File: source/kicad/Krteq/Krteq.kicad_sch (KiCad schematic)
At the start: 137 parts, among them J71 OLED 128x32, SW1 Switch, SW10 Switch, SW11 Switch, SW12 Switch, SW13 Switch, SW14 Switch, SW15 Switch, SW16 Switch, SW17 Switch, SW18 Switch, SW19 Switch, SW2 Switch, SW20 Switch, SW21 Switch, SW22 Switch, SW23 Switch, SW24 Switch, SW25 Switch, SW26 Switch, SW27 Switch, SW28 Switch, SW29 Switch, SW3 Switch, SW30 Switch, SW31 Switch, SW32 Switch, SW33 Switch, SW34 Switch, SW35 Switch, SW36 Switch, SW37 Switch, SW38 Switch, SW39 Switch, SW4 Switch, SW40 Switch, SW41 Switch, SW42 Switch, SW43 Switch, SW44 Switch, SW45 Switch, SW46 Switch, SW47 Switch, SW48 Switch, SW49 Switch, SW5 Switch, SW50 Switch, SW51 Switch, SW52 Switch, SW53 Switch, SW54 Switch, SW55 Switch, SW56 Switch, SW57 Switch, SW58 Switch, SW59 Switch, SW6 Switch, SW60 Switch, SW61 Switch, SW7 Switch, SW8 Switch, SW9 Switch, U71 IS31FL3733-QF

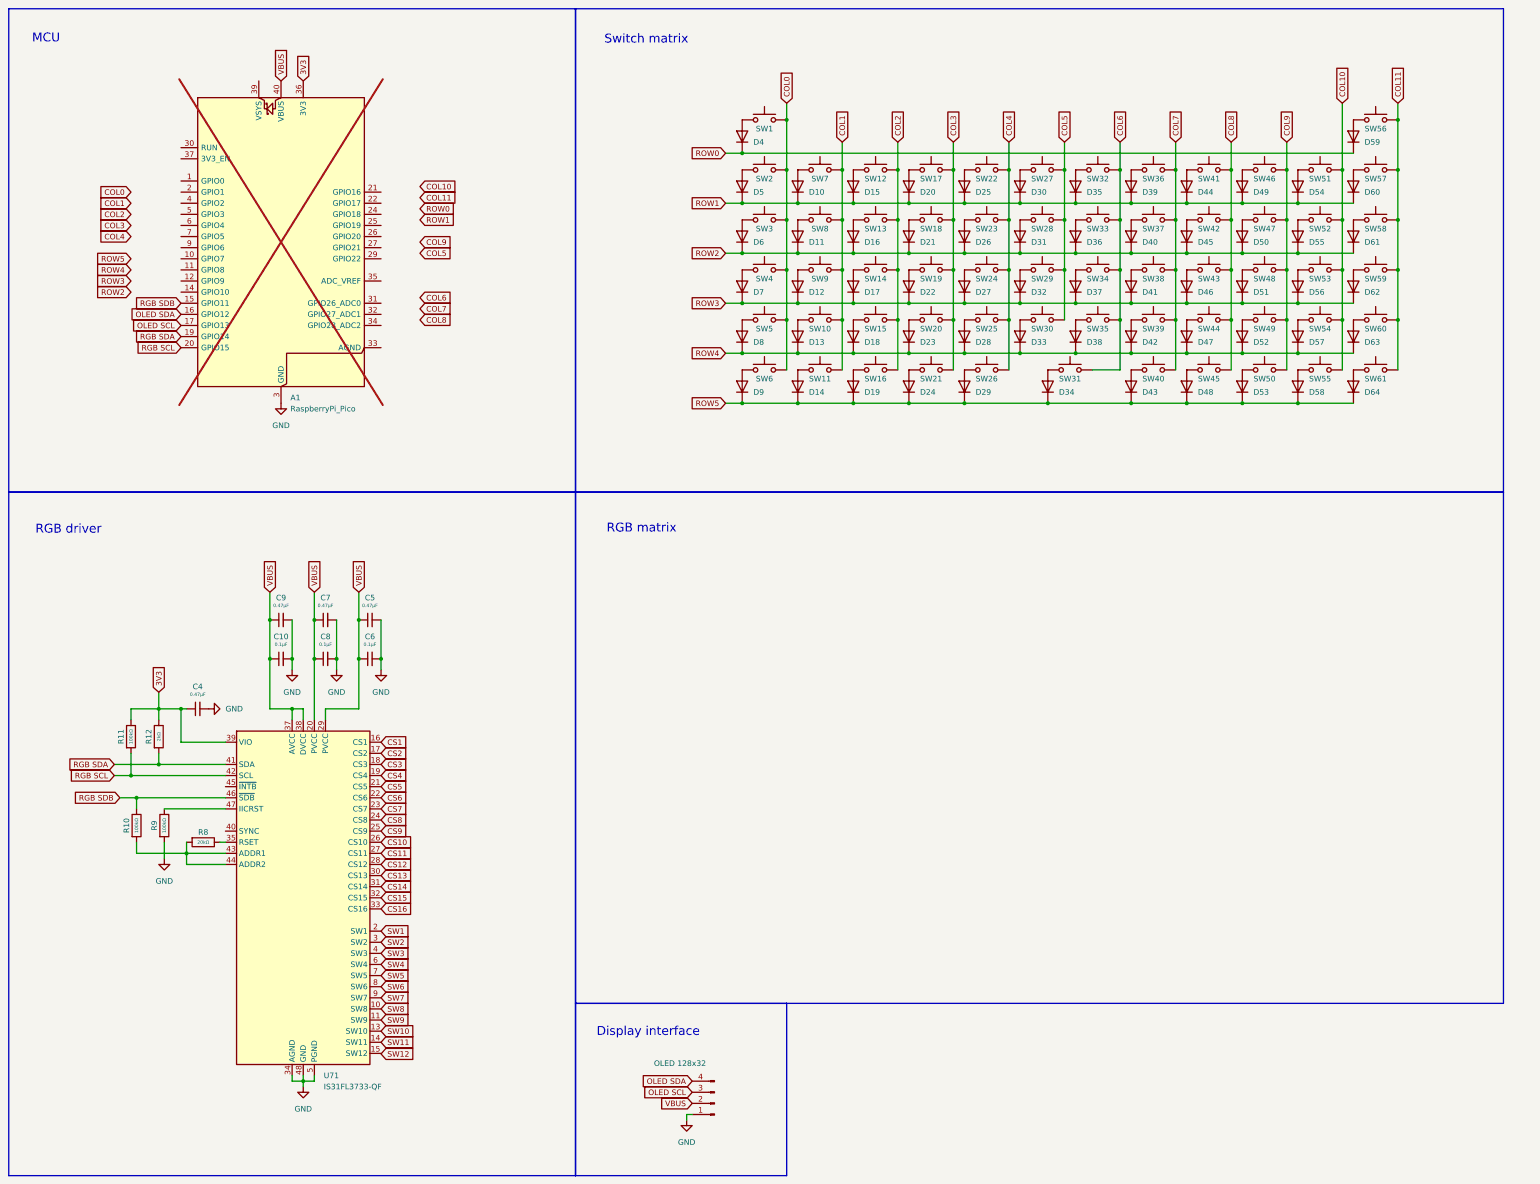
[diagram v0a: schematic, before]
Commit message: update
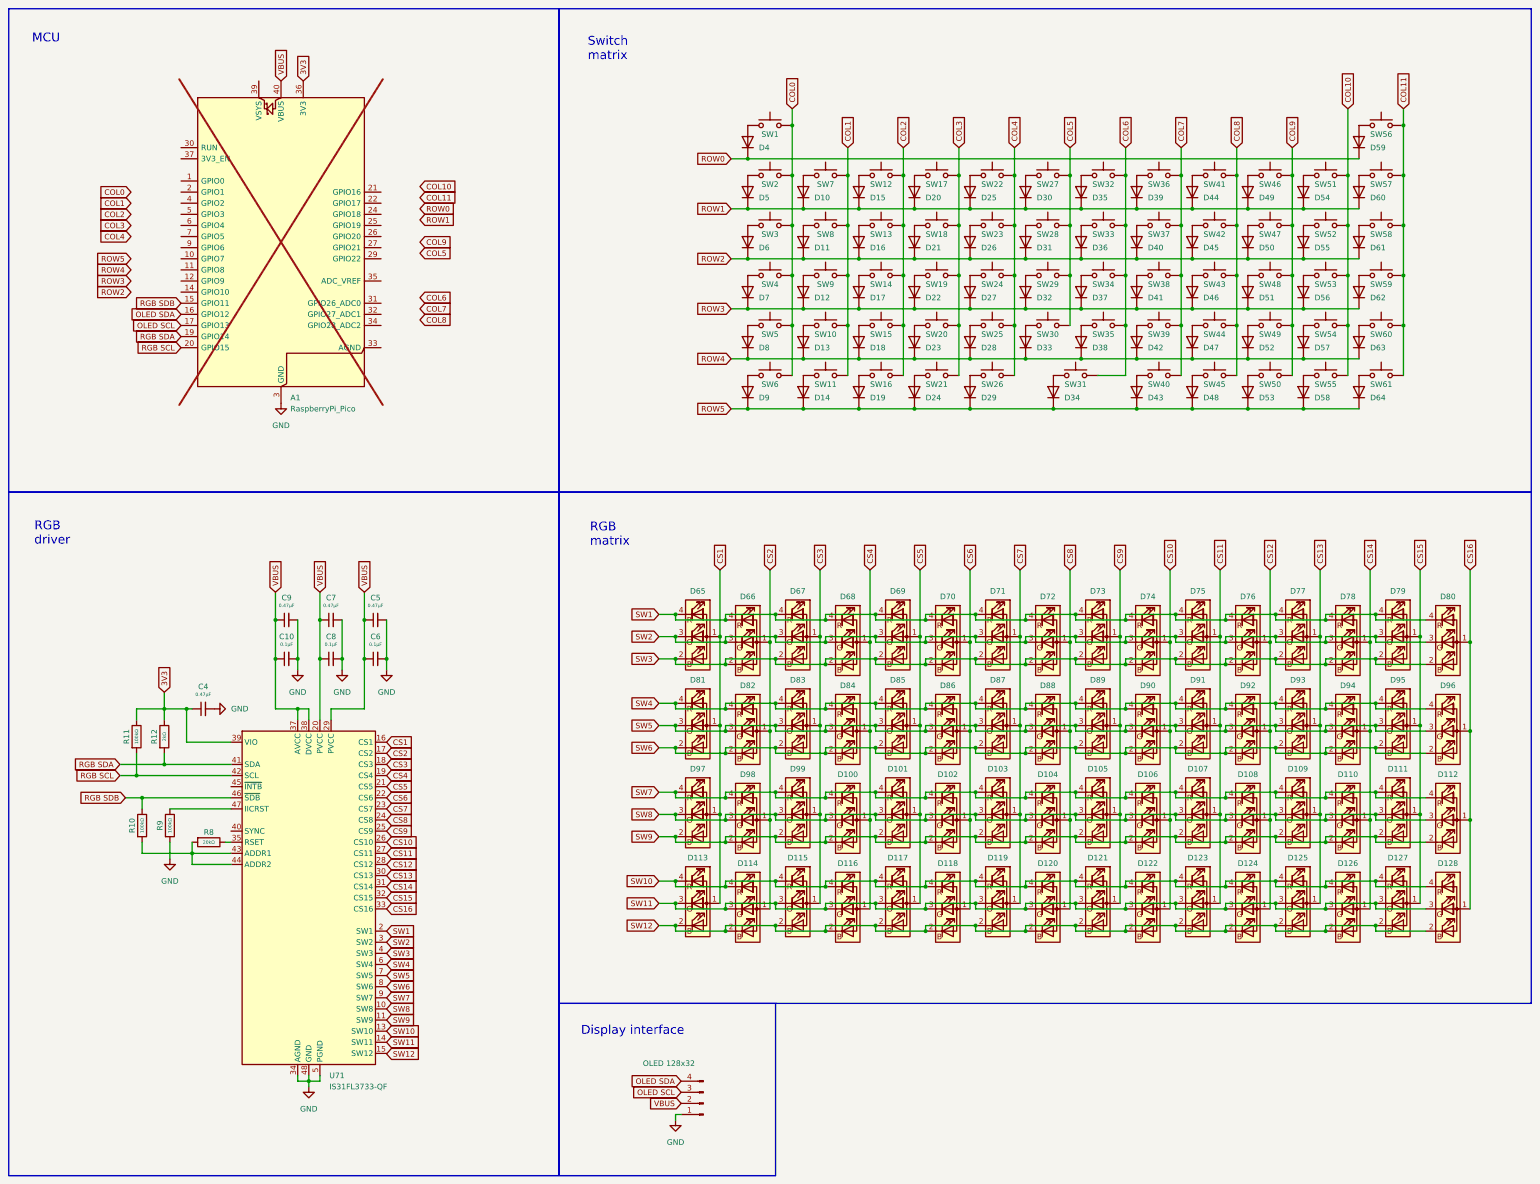
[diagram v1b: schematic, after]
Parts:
- added D100, D101, D102, D103, D104, D105, D106, D107, D108, D109, D110, D111, D112, D113, D114, D115, D116, D117, D118, D119, D120, D121, D122, D123, D124, D125, D126, D127, D128, D65, D66, D67, D68, D69, D70, D71, D72, D73, D74, D75, D76, D77, D78, D79, D80, D81, D82, D83, D84, D85, D86, D87, D88, D89, D90, D91, D92, D93, D94, D95, D96, D97, D98, D99: LED_ABGR, symbol Device:LED_ABGR
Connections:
- net CS1: now also D113.1 (A), D65.1 (A), D81.1 (A), D97.1 (A)
- net CS10: now also D106.1 (A), D122.1 (A), D74.1 (A), D90.1 (A)
- net CS11: now also D107.1 (A), D123.1 (A), D75.1 (A), D91.1 (A)
- net CS12: now also D108.1 (A), D124.1 (A), D76.1 (A), D92.1 (A)
- net CS13: now also D109.1 (A), D125.1 (A), D77.1 (A), D93.1 (A)
- net CS14: now also D110.1 (A), D126.1 (A), D78.1 (A), D94.1 (A)
- net CS15: now also D111.1 (A), D127.1 (A), D79.1 (A), D95.1 (A)
- net CS16: now also D112.1 (A), D128.1 (A), D80.1 (A), D96.1 (A)
- net CS2: now also D114.1 (A), D66.1 (A), D82.1 (A), D98.1 (A)
- net CS3: now also D115.1 (A), D67.1 (A), D83.1 (A), D99.1 (A)
- net CS4: now also D100.1 (A), D116.1 (A), D68.1 (A), D84.1 (A)
- net CS5: now also D101.1 (A), D117.1 (A), D69.1 (A), D85.1 (A)
- net CS6: now also D102.1 (A), D118.1 (A), D70.1 (A), D86.1 (A)
- net CS7: now also D103.1 (A), D119.1 (A), D71.1 (A), D87.1 (A)
- net CS8: now also D104.1 (A), D120.1 (A), D72.1 (A), D88.1 (A)
- net CS9: now also D105.1 (A), D121.1 (A), D73.1 (A), D89.1 (A)
- net SW1: now also D65.4 (RK), D66.4 (RK), D67.4 (RK), D68.4 (RK), D69.4 (RK), D70.4 (RK), D71.4 (RK), D72.4 (RK), D73.4 (RK), D74.4 (RK), D75.4 (RK), D76.4 (RK), D77.4 (RK), D78.4 (RK), D79.4 (RK), D80.4 (RK)
- net SW10: now also D113.4 (RK), D114.4 (RK), D115.4 (RK), D116.4 (RK), D117.4 (RK), D118.4 (RK), D119.4 (RK), D120.4 (RK), D121.4 (RK), D122.4 (RK), D123.4 (RK), D124.4 (RK), D125.4 (RK), D126.4 (RK), D127.4 (RK), D128.4 (RK)
- net SW11: now also D113.3 (GK), D114.3 (GK), D115.3 (GK), D116.3 (GK), D117.3 (GK), D118.3 (GK), D119.3 (GK), D120.3 (GK), D121.3 (GK), D122.3 (GK), D123.3 (GK), D124.3 (GK), D125.3 (GK), D126.3 (GK), D127.3 (GK), D128.3 (GK)
- net SW12: now also D113.2 (BK), D114.2 (BK), D115.2 (BK), D116.2 (BK), D117.2 (BK), D118.2 (BK), D119.2 (BK), D120.2 (BK), D121.2 (BK), D122.2 (BK), D123.2 (BK), D124.2 (BK), D125.2 (BK), D126.2 (BK), D127.2 (BK), D128.2 (BK)
- net SW2: now also D65.3 (GK), D66.3 (GK), D67.3 (GK), D68.3 (GK), D69.3 (GK), D70.3 (GK), D71.3 (GK), D72.3 (GK), D73.3 (GK), D74.3 (GK), D75.3 (GK), D76.3 (GK), D77.3 (GK), D78.3 (GK), D79.3 (GK), D80.3 (GK)
- net SW3: now also D65.2 (BK), D66.2 (BK), D67.2 (BK), D68.2 (BK), D69.2 (BK), D70.2 (BK), D71.2 (BK), D72.2 (BK), D73.2 (BK), D74.2 (BK), D75.2 (BK), D76.2 (BK), D77.2 (BK), D78.2 (BK), D79.2 (BK), D80.2 (BK)
- net SW4: now also D81.4 (RK), D82.4 (RK), D83.4 (RK), D84.4 (RK), D85.4 (RK), D86.4 (RK), D87.4 (RK), D88.4 (RK), D89.4 (RK), D90.4 (RK), D91.4 (RK), D92.4 (RK), D93.4 (RK), D94.4 (RK), D95.4 (RK), D96.4 (RK)
- net SW5: now also D81.3 (GK), D82.3 (GK), D83.3 (GK), D84.3 (GK), D85.3 (GK), D86.3 (GK), D87.3 (GK), D88.3 (GK), D89.3 (GK), D90.3 (GK), D91.3 (GK), D92.3 (GK), D93.3 (GK), D94.3 (GK), D95.3 (GK), D96.3 (GK)
- net SW6: now also D81.2 (BK), D82.2 (BK), D83.2 (BK), D84.2 (BK), D85.2 (BK), D86.2 (BK), D87.2 (BK), D88.2 (BK), D89.2 (BK), D90.2 (BK), D91.2 (BK), D92.2 (BK), D93.2 (BK), D94.2 (BK), D95.2 (BK), D96.2 (BK)
- net SW7: now also D100.4 (RK), D101.4 (RK), D102.4 (RK), D103.4 (RK), D104.4 (RK), D105.4 (RK), D106.4 (RK), D107.4 (RK), D108.4 (RK), D109.4 (RK), D110.4 (RK), D111.4 (RK), D112.4 (RK), D97.4 (RK), D98.4 (RK), D99.4 (RK)
- net SW8: now also D100.3 (GK), D101.3 (GK), D102.3 (GK), D103.3 (GK), D104.3 (GK), D105.3 (GK), D106.3 (GK), D107.3 (GK), D108.3 (GK), D109.3 (GK), D110.3 (GK), D111.3 (GK), D112.3 (GK), D97.3 (GK), D98.3 (GK), D99.3 (GK)
- net SW9: now also D100.2 (BK), D101.2 (BK), D102.2 (BK), D103.2 (BK), D104.2 (BK), D105.2 (BK), D106.2 (BK), D107.2 (BK), D108.2 (BK), D109.2 (BK), D110.2 (BK), D111.2 (BK), D112.2 (BK), D97.2 (BK), D98.2 (BK), D99.2 (BK)
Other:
- moved on the sheet: C10, C4, C5, C6, C7, C8, C9, D10, D11, D12, D13, D14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

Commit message: update
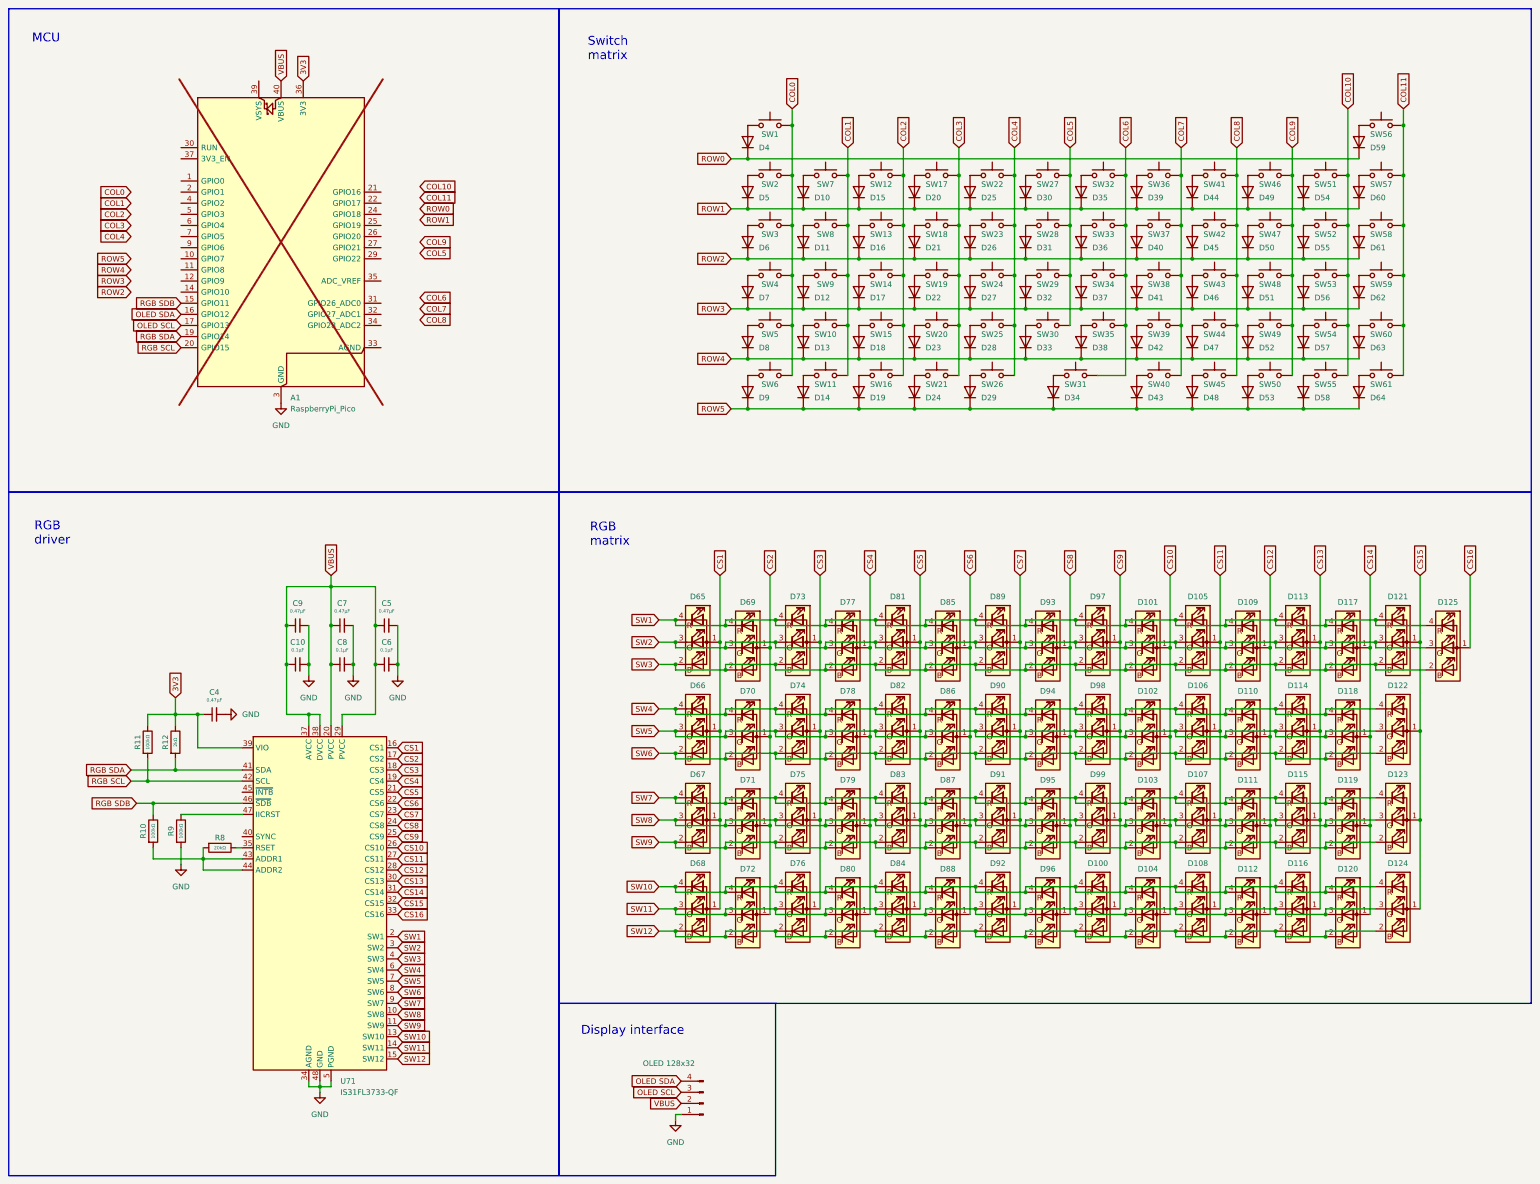
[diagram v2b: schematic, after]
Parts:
- removed D112, D128, D96: LED_ABGR, symbol Device:LED_ABGR
- renumbered D121 to D100, D74 to D101, D90 to D102, D106 to D103, D122 to D104, D75 to D105, D91 to D106, D123 to D108, D76 to D109, D92 to D110, D108 to D111, D124 to D112, D77 to D113, D93 to D114, D109 to D115, D125 to D116, D78 to D117, D94 to D118, D110 to D119, D126 to D120, D79 to D121, D95 to D122, D111 to D123, D127 to D124, D80 to D125, D81 to D66, D97 to D67, D113 to D68, D66 to D69, D82 to D70, D98 to D71, D114 to D72, D67 to D73, D83 to D74, D99 to D75, D115 to D76, D68 to D77, D84 to D78, D100 to D79, D116 to D80, D69 to D81, D85 to D82, D101 to D83, D117 to D84, D70 to D85, D102 to D87, D118 to D88, D71 to D89, D87 to D90, D103 to D91, D119 to D92, D72 to D93, D88 to D94, D104 to D95, D120 to D96, D73 to D97, D89 to D98, D105 to D99
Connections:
- net SW12: now also U71.15 (SW12)
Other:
- moved on the sheet: C10, C4, C5, C6, C7, C8, C9, D100, D101, D102, D103, D104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
